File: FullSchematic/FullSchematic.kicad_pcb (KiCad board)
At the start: 2 copper layers, 100 x 100 mm, 85 parts, among them IC1 TTP223E-BA6, J1 USB_B_Micro, J2 TP4056, J3 Conn_01x03_Pin, J4 Conn_01x03_Pin, J5 Conn_01x03_Pin, P1 Touch Pad, Q1 IRLML6402, Q2 IRLML6402, Q3 IRLML6402, Q4 2N7002, U1 LM1117-3.3, U2 CH340C, U3 24LC64, U4 STM32F051C6T6, U5 OP184, U6 CJ432

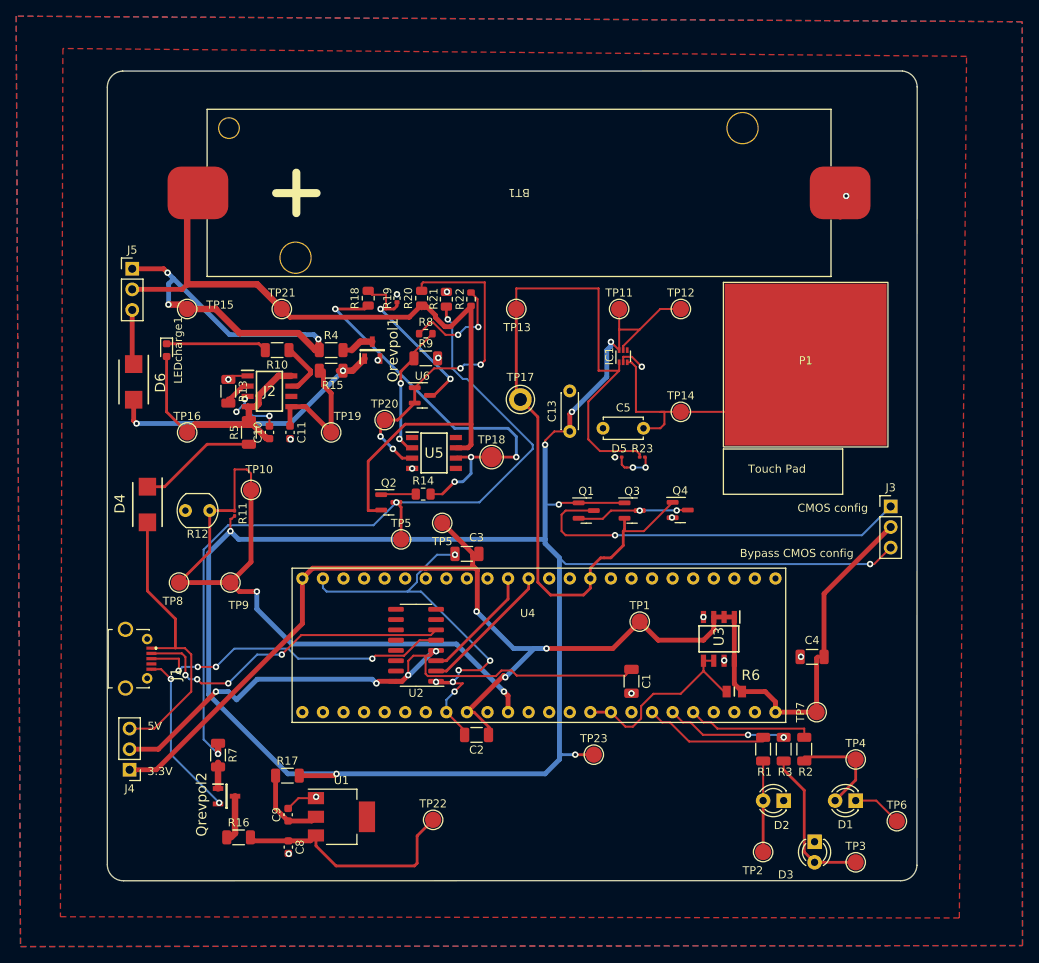
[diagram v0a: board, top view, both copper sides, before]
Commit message: generated files
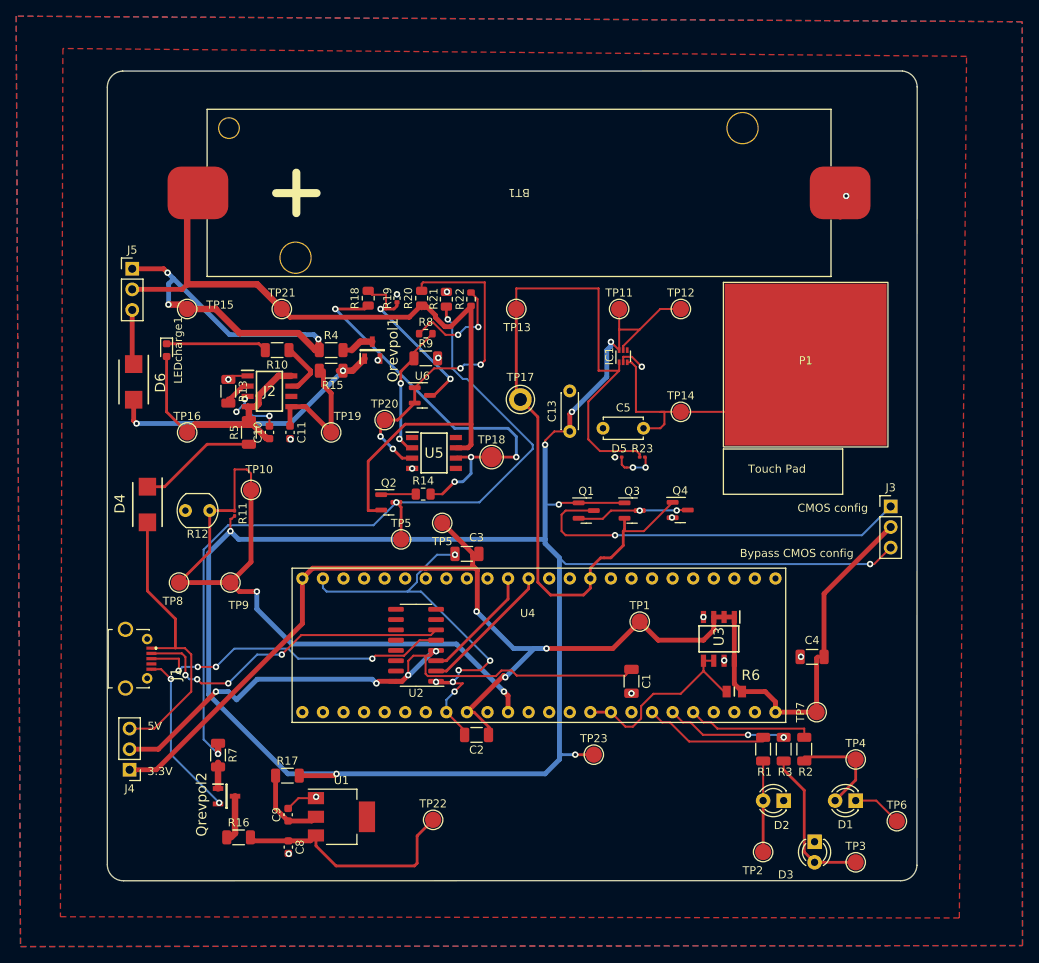
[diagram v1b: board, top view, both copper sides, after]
